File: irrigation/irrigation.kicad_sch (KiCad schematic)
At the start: 37 parts, among them J1 24V Jmp, J10 24V, J11 25%, J12 50%, J13 75%, J14 100%, J15 100%, J16 100%, J17 Pump, J2 Power, J3 Power, J4 Power, J5 Power, J6 Power, J7 Power, J8 0V Jmp, J9 Empty, K1 PLC-RPT-24DC/21, K2 PLC-RPT-24DC/21, M1 Pump, SW1 Well Empty, SW2 100% Full, SW3 25% Full, SW4 50% Full, SW5 75% Full, U1 MPPT-Charger

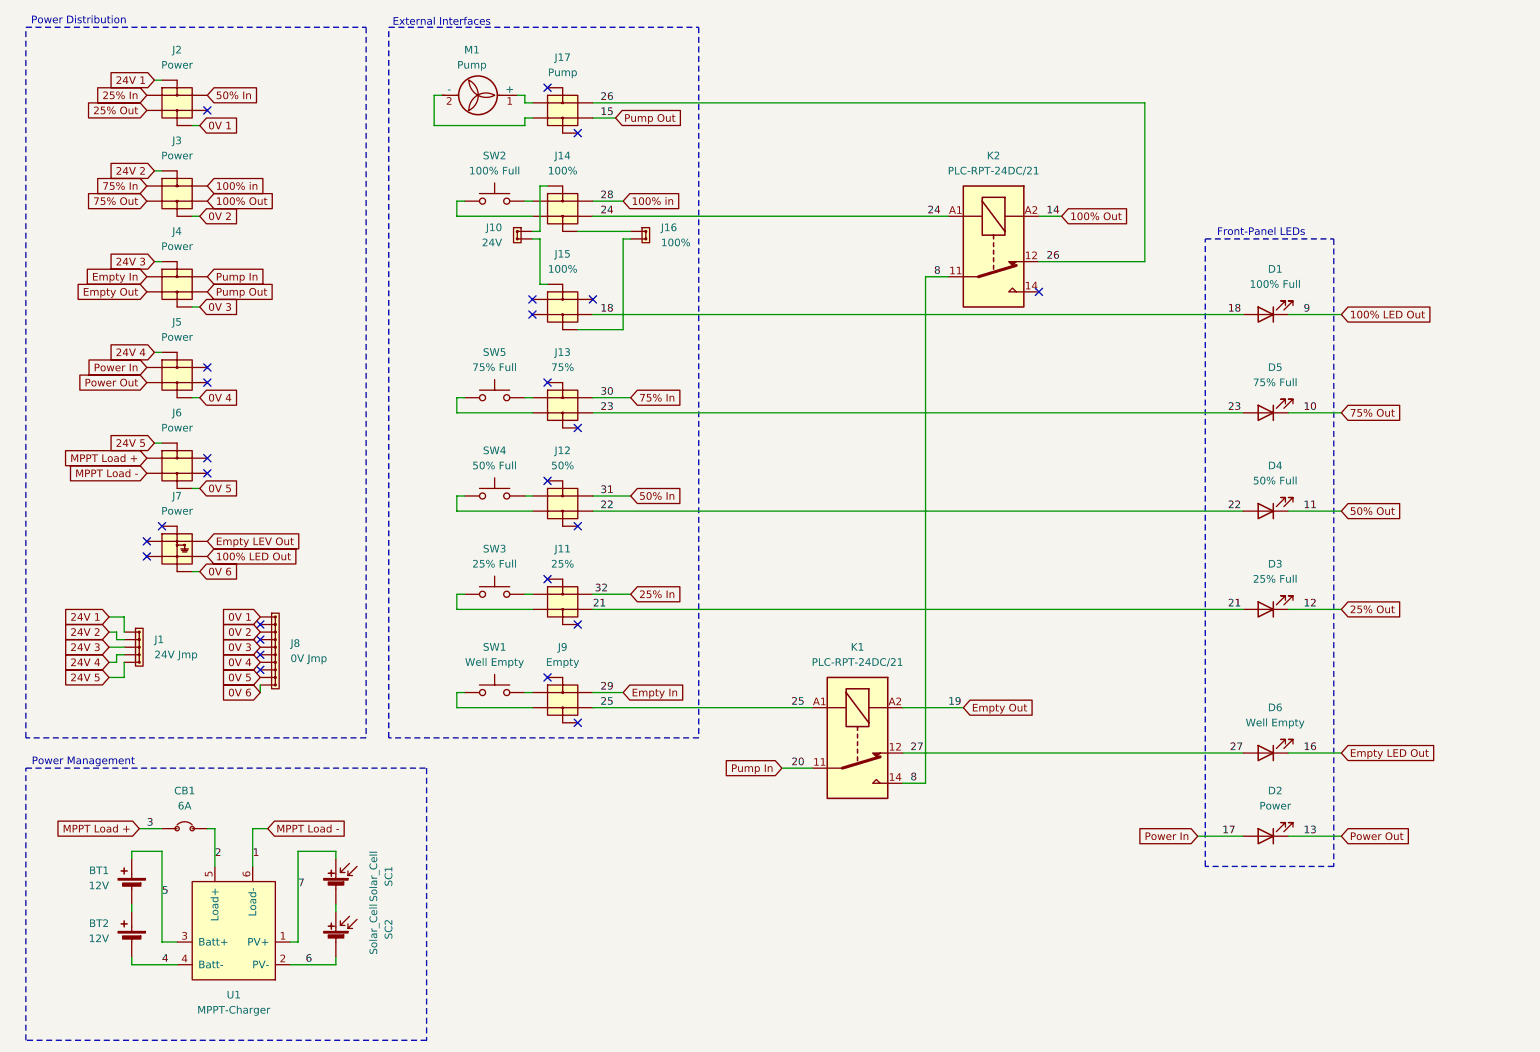
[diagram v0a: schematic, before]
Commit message: Organized.
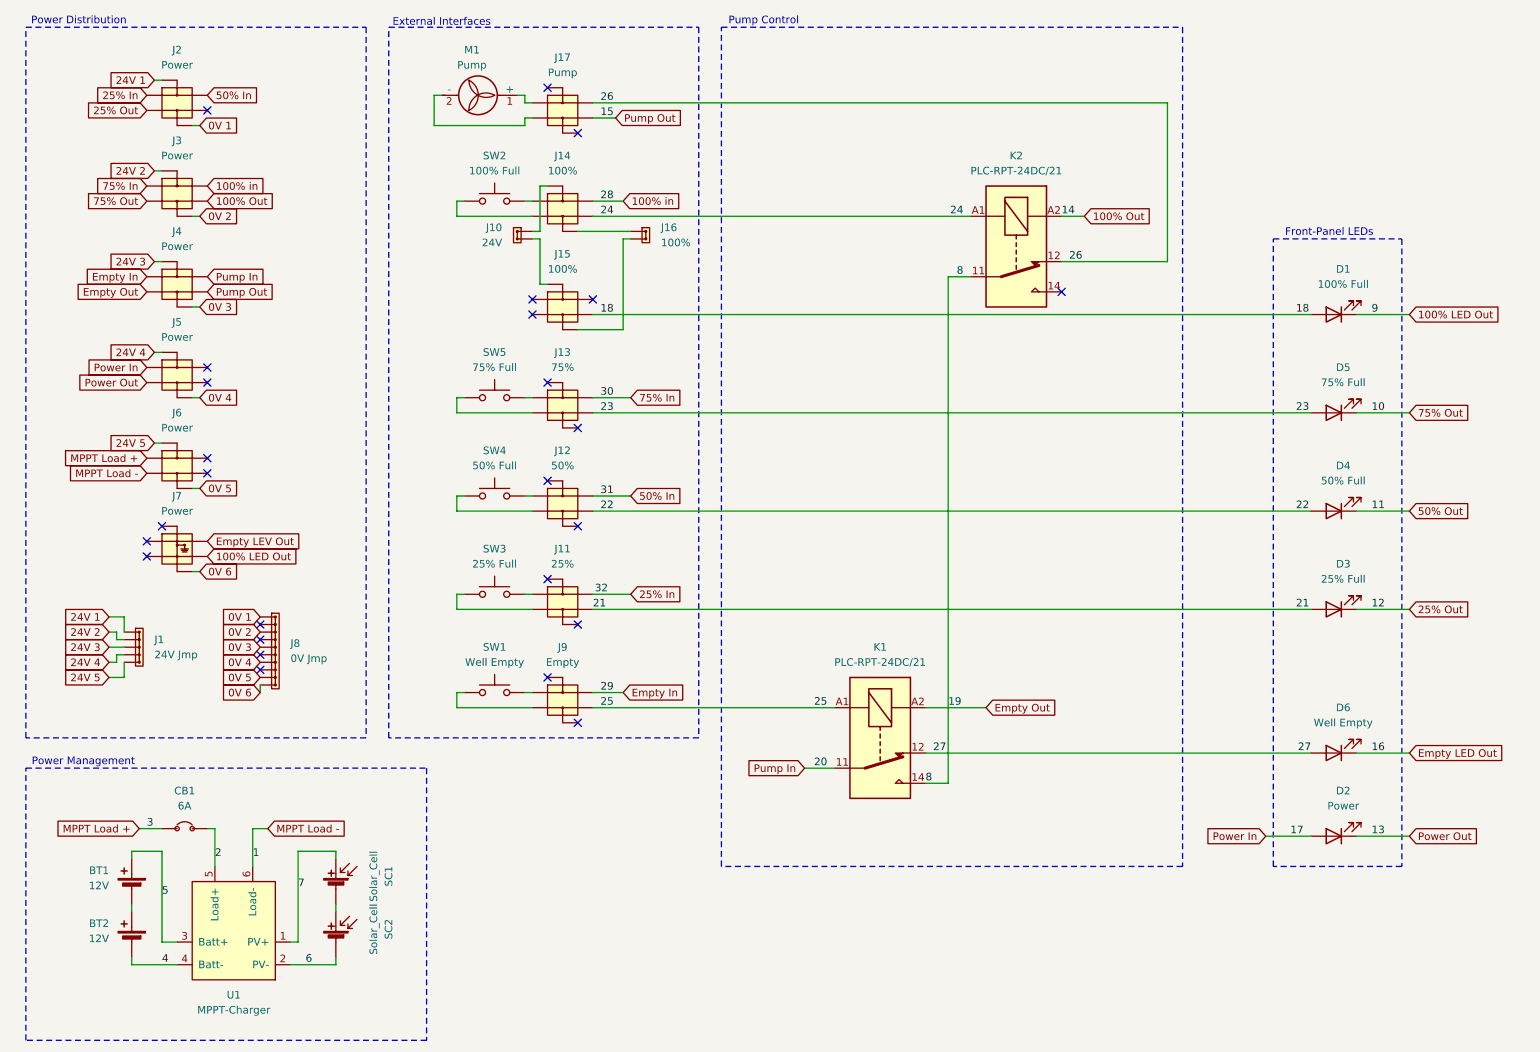
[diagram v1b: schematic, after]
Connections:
- net 8 is gone; now on net Empty Out: K1.14, K2.11
- net at J10.: now also J15.; no longer J14.
- net at J16.: now also J15.; no longer J14.
- new net: J10., J14.
- new net: J14., J16.
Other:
- note added: "Pump Control"
- moved on the sheet: D1, D2, D3, D4, D5, D6, K1, K2
